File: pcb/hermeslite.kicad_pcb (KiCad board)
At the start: 4 copper layers, 49.9 x 49.9 mm, 71 parts, among them CN1 MEC6-140_CONNECTOR_BEMICRO, CN2 PCIE, CN4 SATA22, J1 0, J2 0, J3 0, J4 0, J5 0, P0 CONN_1, P12 CONN_1, P3 CONN_1, P5 CONN_1, U1 AD9866BCPZ, U2 EEPROM, X1 61.440

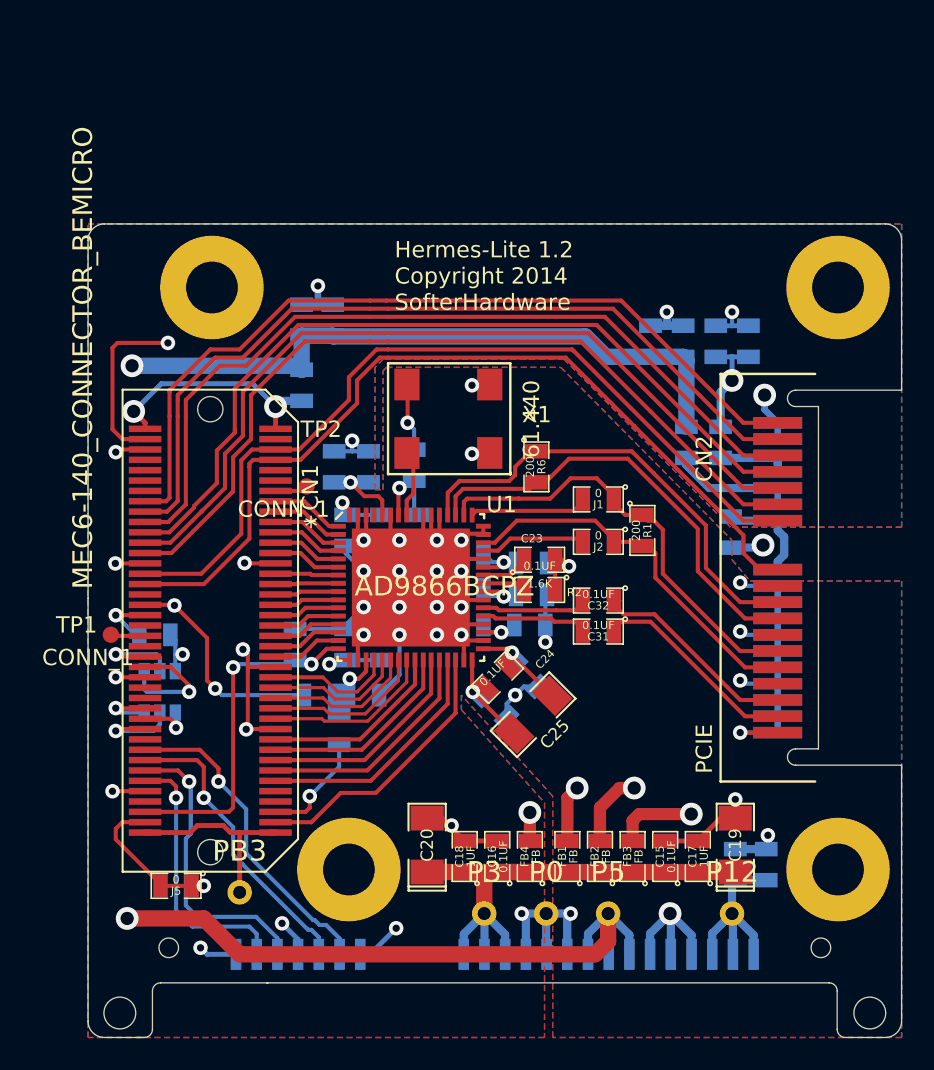
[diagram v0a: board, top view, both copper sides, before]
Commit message: Version 1.2 for review
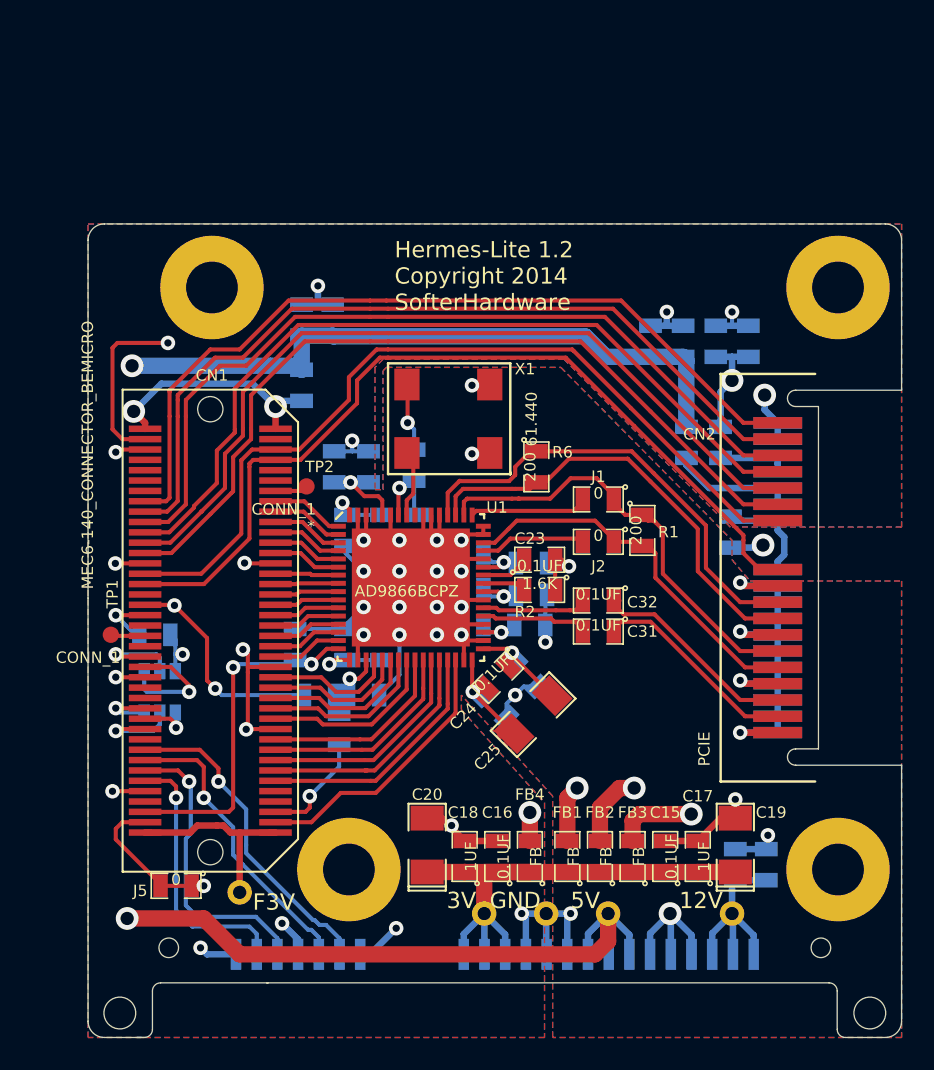
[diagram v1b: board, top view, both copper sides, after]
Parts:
- P3: value CONN_1 -> 3V
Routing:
- net GND: track 288.1 -> 299.9 mm
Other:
- board text added: "12V"
- board text added: "3V"
- board text added: "5V"
- board text added: "F3V"
- board text added: "GND"
